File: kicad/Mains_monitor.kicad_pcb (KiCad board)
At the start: 2 copper layers, 99.5 x 99.5 mm, 35 parts, among them J1 Screw_Terminal_01x02, J2 Screw_Terminal_01x02, K1 SANYOU_SRD_Form_C, Q1 NPN, U1 HLW8032

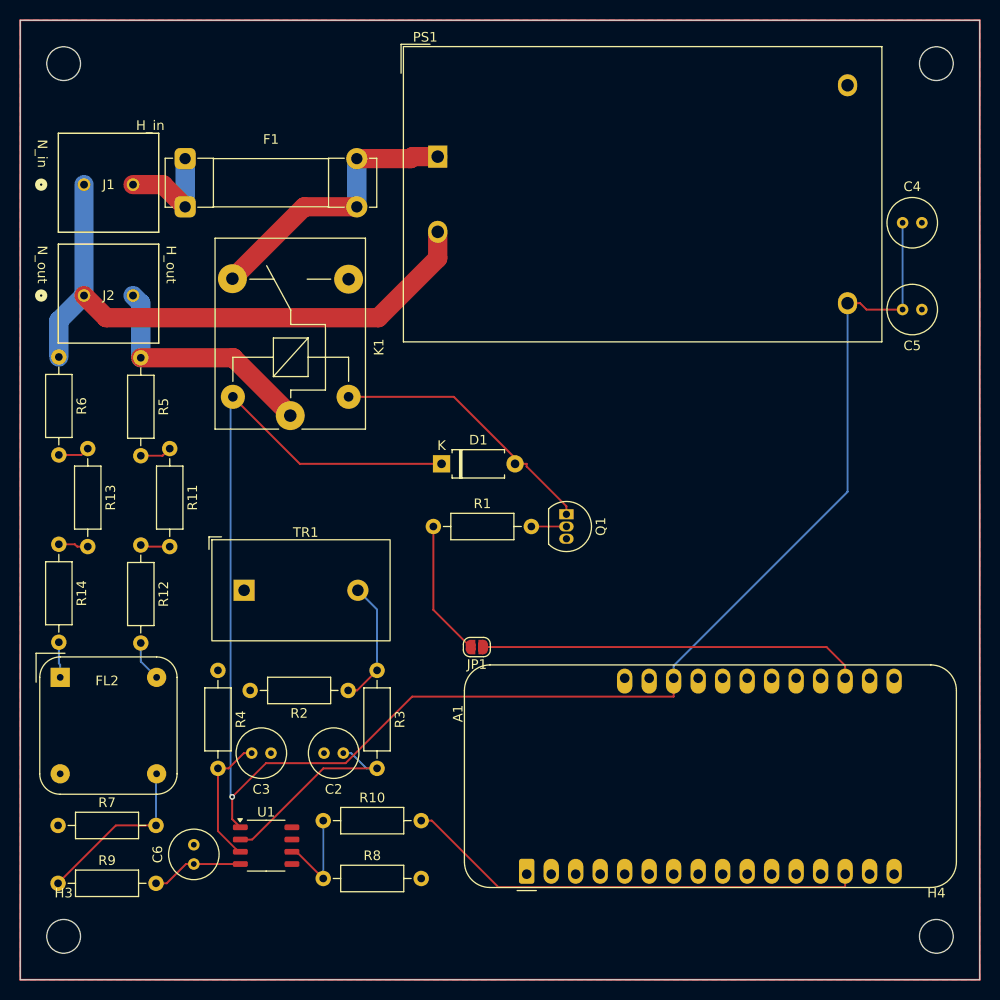
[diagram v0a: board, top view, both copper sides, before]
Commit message: backup files
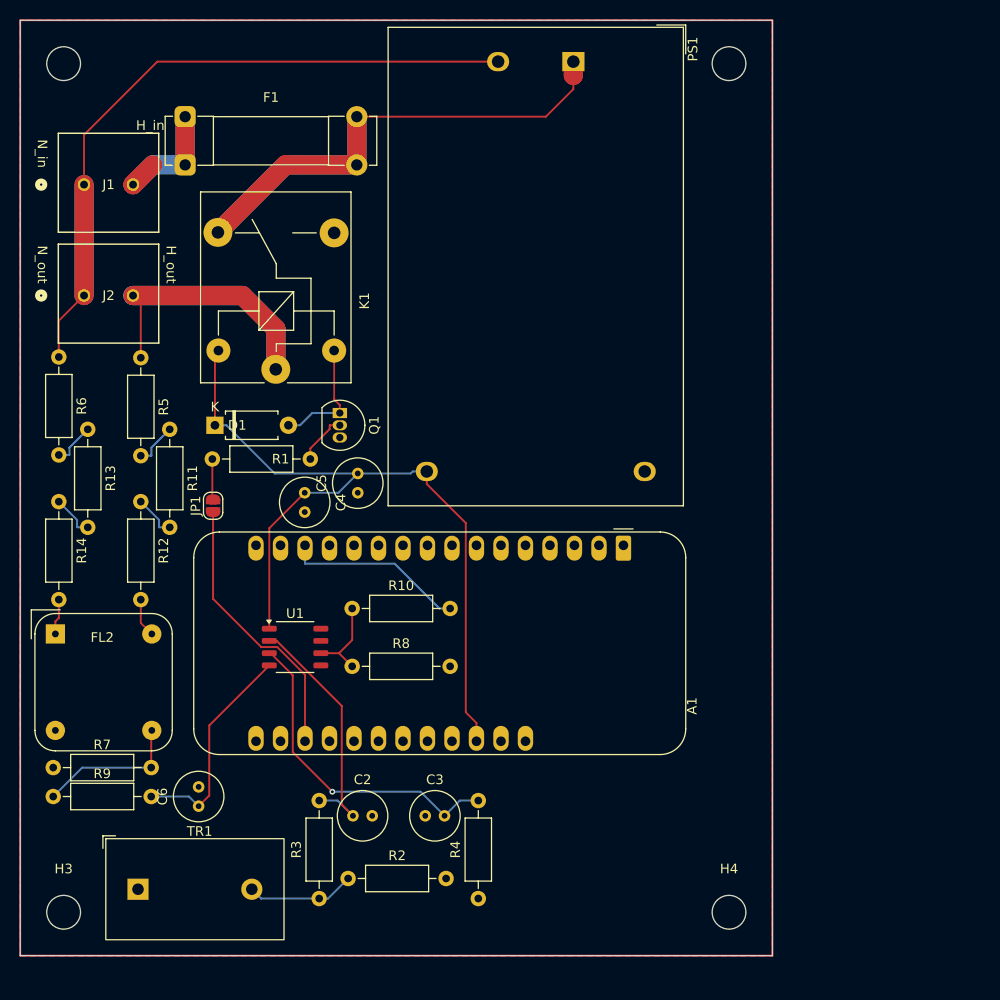
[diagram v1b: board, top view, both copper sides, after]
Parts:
- moved C4 68.0 mm to (120.0, 94.0), turned to -90 degrees
- moved C5 61.5 mm to (125.5, 94.0), turned to 90 degrees
- moved R4 35.9 mm to (138.0, 136.1), turned to 90 degrees
- moved A1 35.5 mm to (153.1, 99.4), turned to -90 degrees
- moved TR1 32.9 mm to (102.7, 135.1)
- moved JP1 31.0 mm to (110.5, 95.3), turned to 90 degrees
- moved Q1 25.7 mm to (123.6, 85.7)
- moved R3 24.4 mm to (121.5, 136.1), turned to 90 degrees
- moved R1 24.0 mm to (110.4, 90.5)
- moved D1 23.8 mm to (110.7, 87.0)
- moved R10 22.2 mm to (124.9, 106.0)
- moved R8 22.2 mm to (124.9, 112.0)
- moved H4 21.6 mm to (164.0, 137.5)
- moved H2 21.5 mm to (164.0, 49.5)
- moved U1 20.8 mm to (119.0, 110.0)
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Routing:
- net +5V: track 183.0 -> 84.1 mm, vias 1 -> 0
- net AC_H: track 29.5 -> 72.5 mm
- net /DATA_LV: track 48.1 -> 18.9 mm
- net RELAY_OUT: track 24.8 -> 47.7 mm
- net IN: track 13.9 -> 34.0 mm, vias 0 -> 1
- net AC_N: track 61.9 -> 81.7 mm
- net Net-(D1-A): track 28.9 -> 12.6 mm
- net VP: track 9.57 -> 23.0 mm
- net /RLY_CTRL: track 39.6 -> 28.7 mm
- net Net-(J1-Pin_2): track 11.4 -> 22.0 mm
- net Net-(JP1-B): track 14.1 -> 4.23 mm
- net IP: track 21.4 -> 26.3 mm
- net Net-(FL2-Pad4): track 18.0 -> 15.3 mm
- net Net-(Q1-B): track 3.64 -> 5.38 mm
- net Net-(R2-Pad1): track 13.0 -> 11.2 mm
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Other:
- board size 99.5 x 99.5 mm -> 78 x 97 mm
